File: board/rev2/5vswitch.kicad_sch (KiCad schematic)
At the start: 14 parts, among them Q1 Q_NMOS_DGS, U4 TPS259472ARPWR

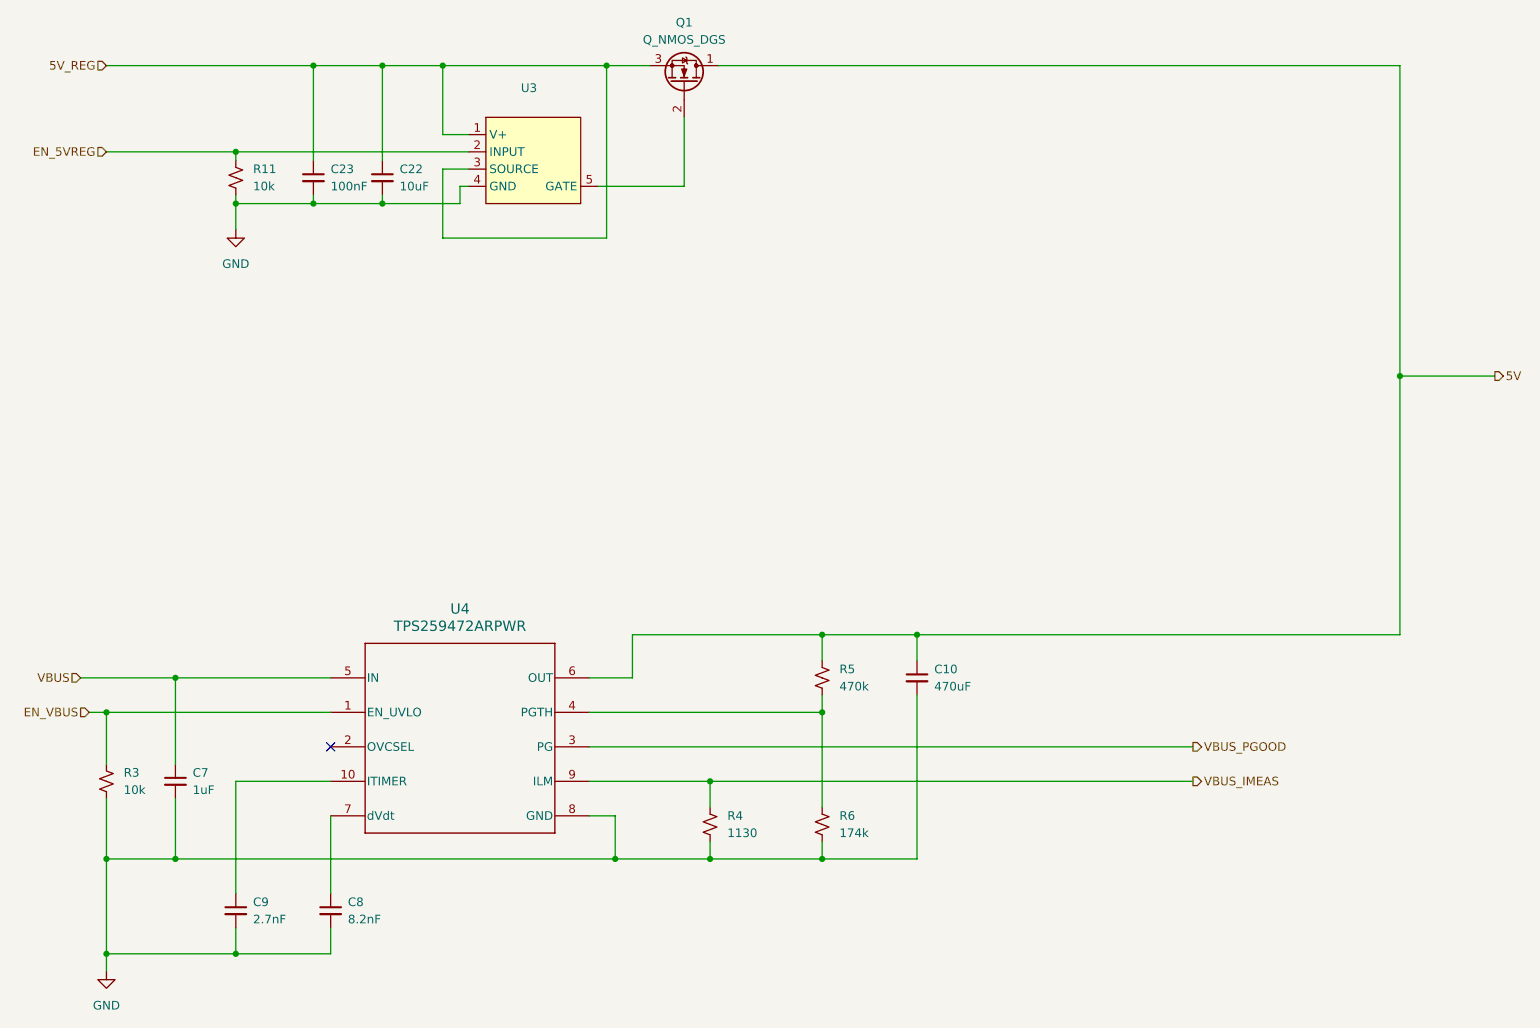
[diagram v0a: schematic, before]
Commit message: More board stuff
(better clk routing, etc.)
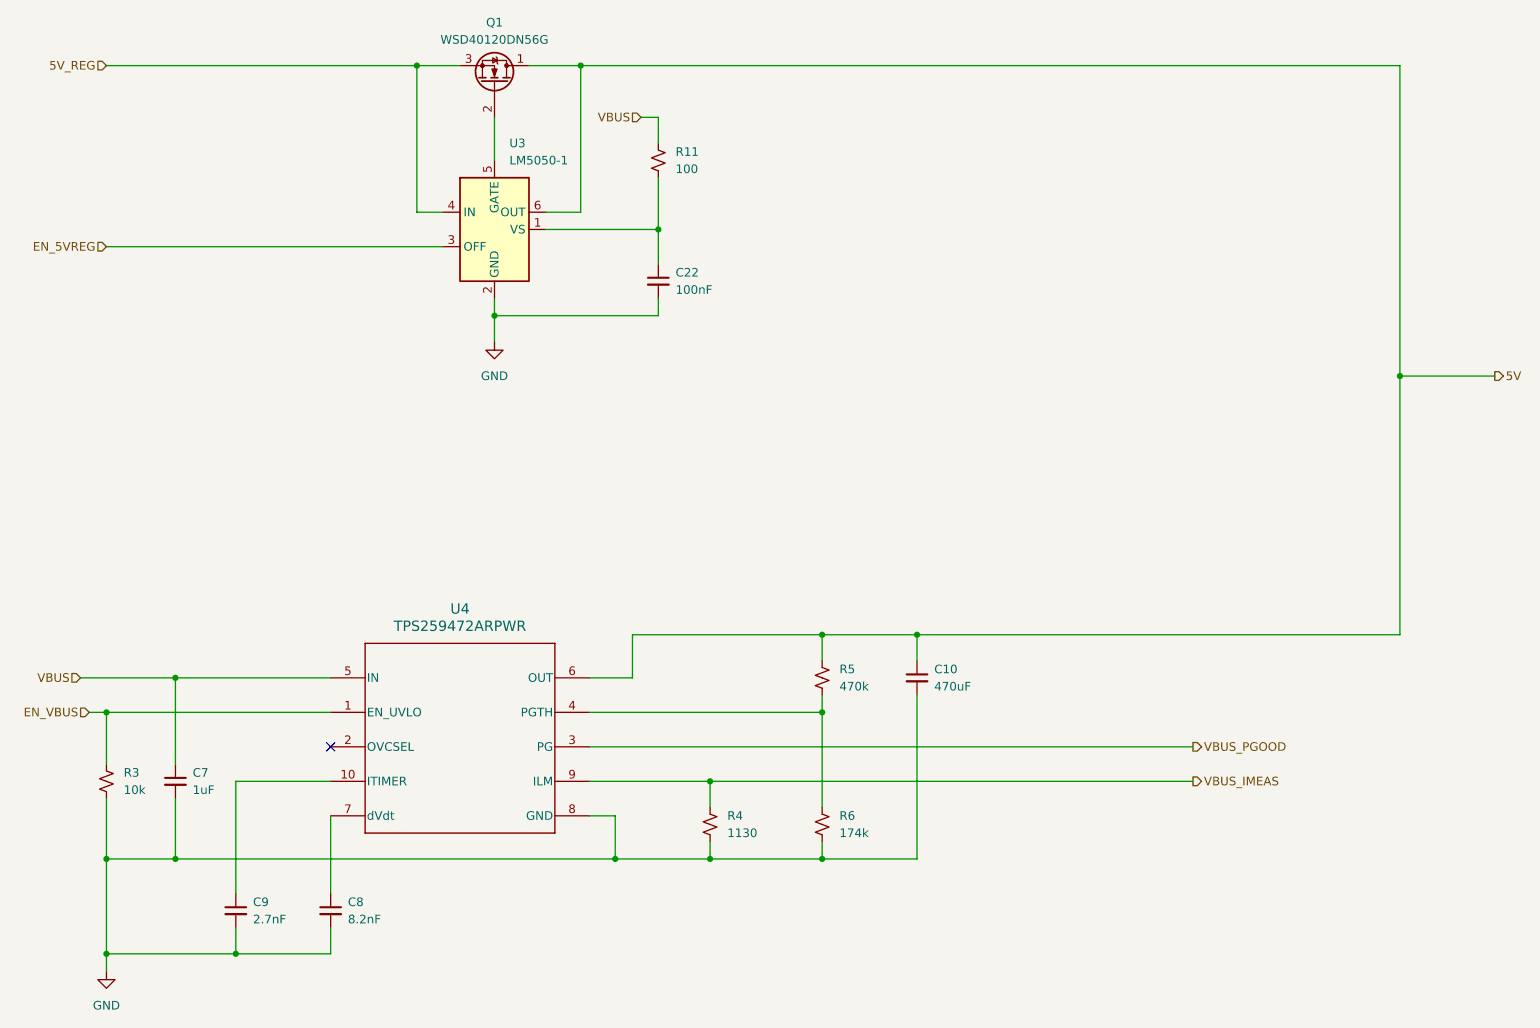
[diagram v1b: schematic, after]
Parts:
- removed C23: 100nF, symbol Device:C_Small
- removed U3: ~, Package_SO:SOP-8_3.9x4.9mm_P1.27mm, symbol WUXI_GateDriver:MX5014S
- added U3: LM5050-1, Package_TO_SOT_SMD:TSOT-23-6, symbol Power_Management:LM5050-1
- C22: value 10uF -> 100nF
- Q1: value Q_NMOS_DGS -> WSD40120DN56G
- R11: value 10k -> 100
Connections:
- net 5V: now also U3.6 (OUT)
- net 5V_REG: now also U3.4 (IN); no longer C22.1
- net EN_5VREG: now also U3.3 (OFF); no longer R11.1
- net GND: now also U3.2 (GND); no longer R11.2
- net VBUS: now also R11.1
- net at Q1.2 (G): now also U3.5 (GATE)
- new net: C22.1, R11.2, U3.1 (VS)
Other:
- moved on the sheet: Q1
